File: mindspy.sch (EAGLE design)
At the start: 39 parts, among them IC1 ADS1298, IC2 TPS7A4901, X1 DF9-31S, X2 STELLARIS-LAUNCHPADSTELLARIS-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

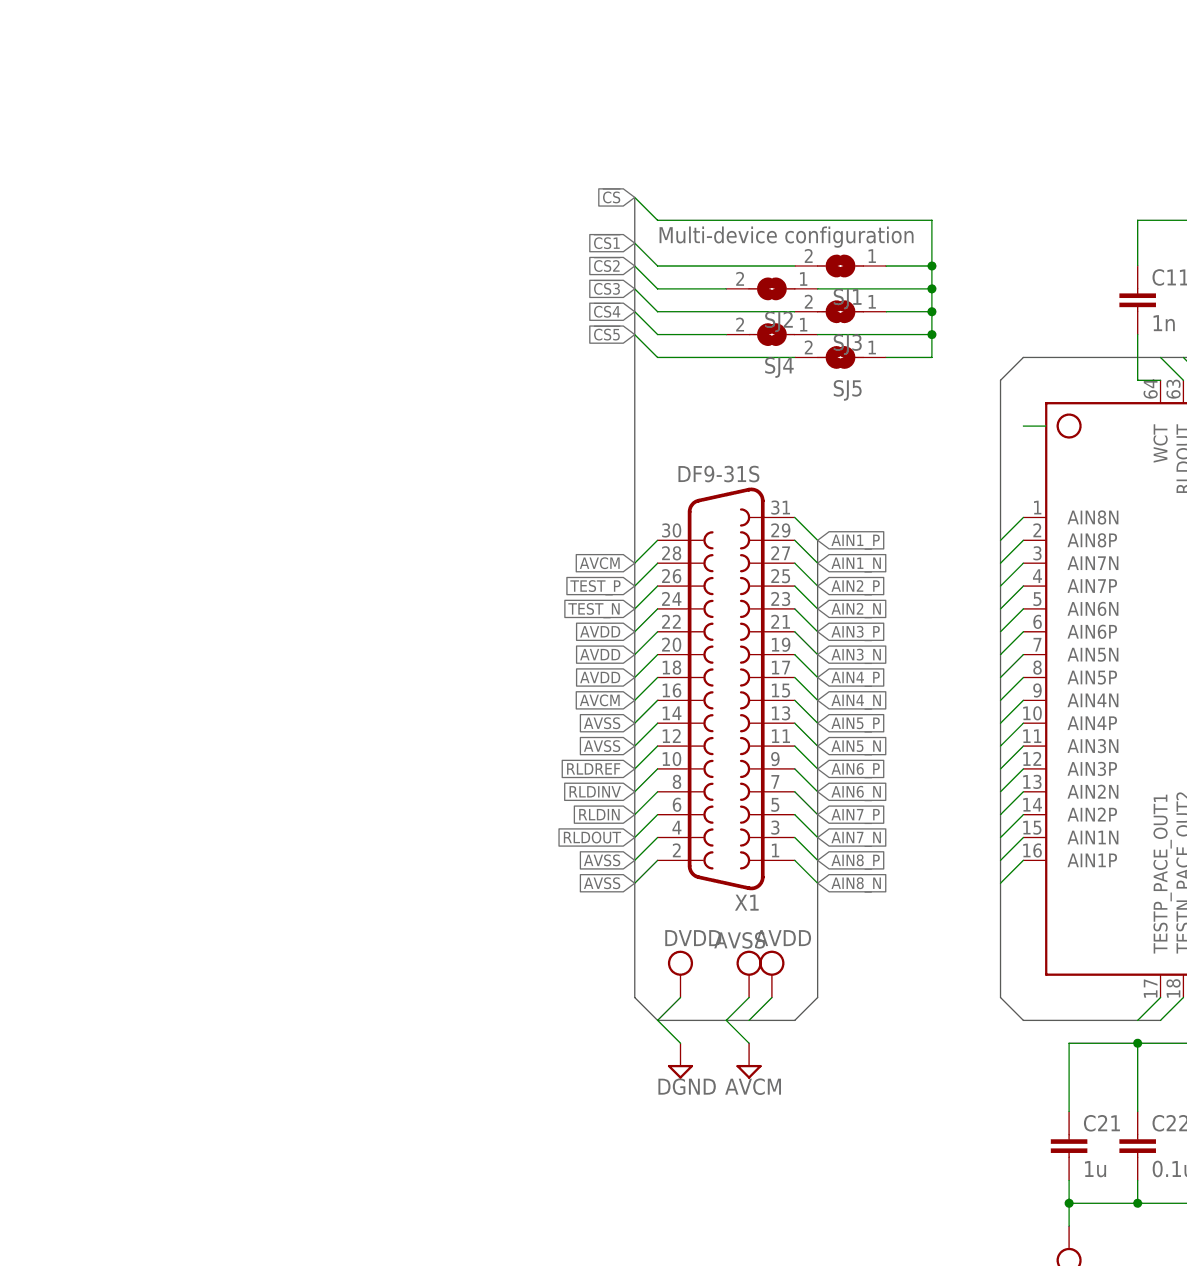
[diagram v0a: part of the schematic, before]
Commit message: almost final
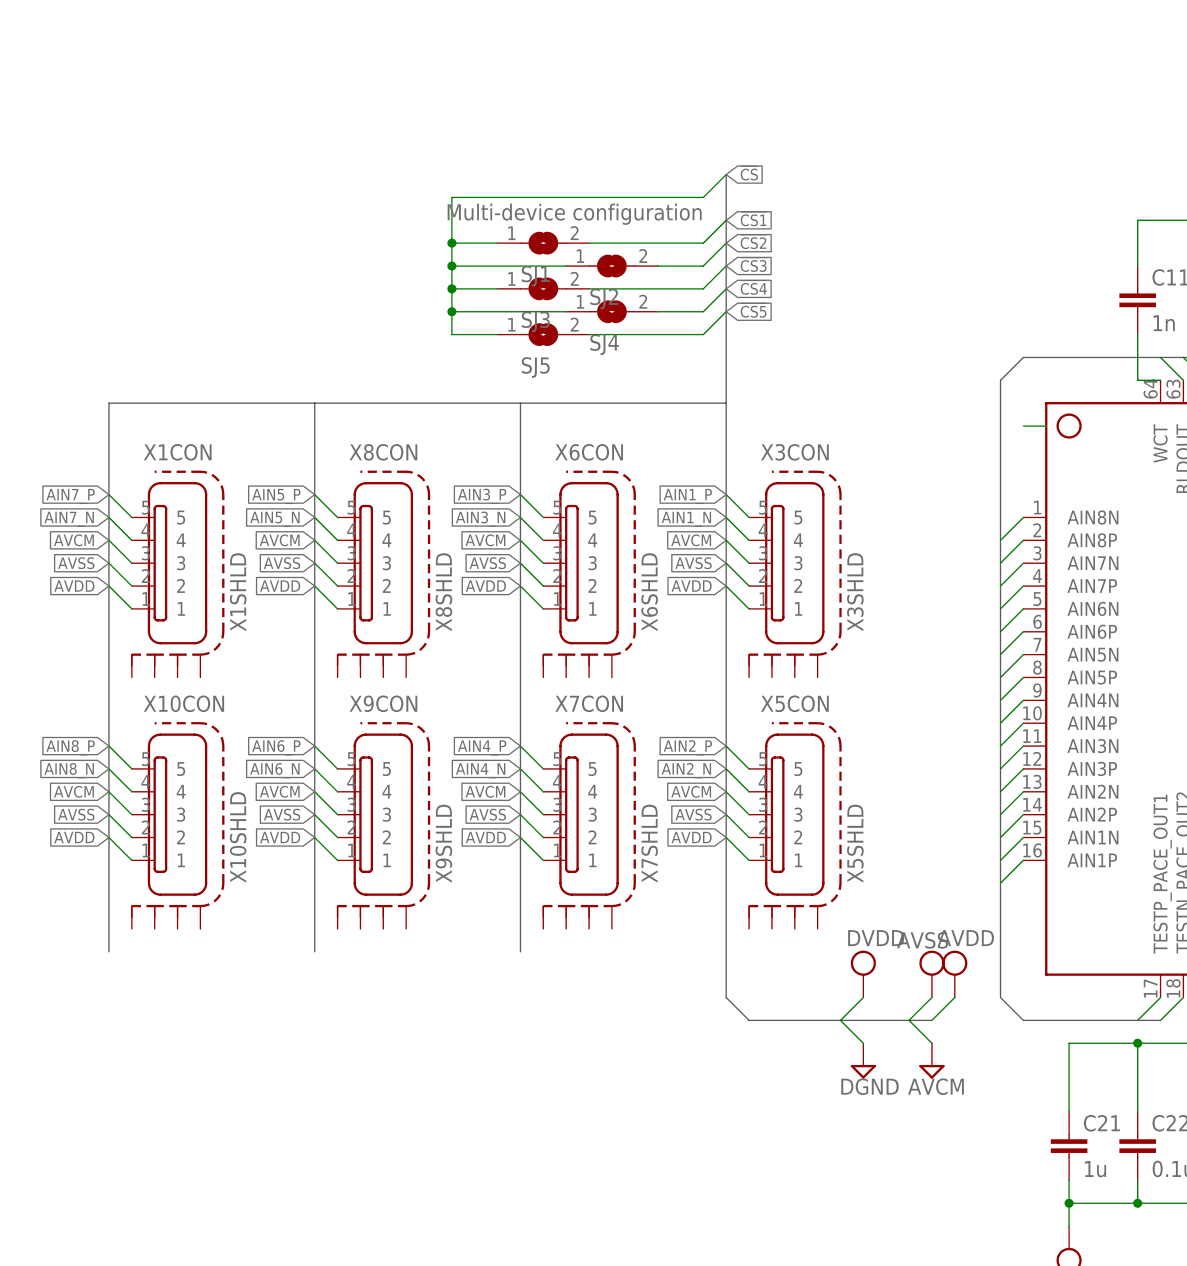
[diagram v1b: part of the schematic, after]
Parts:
- added X10, X3, X5, X6, X7, X8, X9: MICRO-USB-AB-SCHIELD, molex:MICRO-USB-AB-SCHIELD
- X1: value DF9-31S -> MICRO-USB-AB-SCHIELD; device con-hirose:DF9-31S -> molex:MICRO-USB-AB-SCHIELD
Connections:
- net AIN1_N: now also X3CON.4; no longer X1.29
- net AIN1_P: now also X3CON.5; no longer X1.31
- net AIN2_N: now also X5CON.4; no longer X1.25
- net AIN2_P: now also X5CON.5; no longer X1.27
- net AIN3_N: now also X6CON.4; no longer X1.21
- net AIN3_P: now also X6CON.5; no longer X1.23
- net AIN4_N: now also X7CON.4; no longer X1.17
- net AIN4_P: now also X7CON.5; no longer X1.19
- net AIN5_N: now also X8CON.4; no longer X1.13
- net AIN5_P: now also X8CON.5; no longer X1.15
- net AIN6_N: now also X9CON.4; no longer X1.9
- net AIN6_P: now also X9CON.5; no longer X1.11
- net AIN7_N: now also X1CON.4; no longer X1.5
- net AIN7_P: now also X1CON.5; no longer X1.7
- net AIN8_N: now also X10CON.4; no longer X1.1
- net AIN8_P: now also X10CON.5; no longer X1.3
- net AVCM: now also X10CON.3, X1CON.3, X3CON.3, X5CON.3, X6CON.3, X7CON.3, X8CON.3, X9CON.3; no longer X1.18, X1.30
- net AVDD: now also X10CON.1, X1CON.1, X3CON.1, X5CON.1, X6CON.1, X7CON.1, X8CON.1, X9CON.1; no longer X1.20, X1.22, X1.24
- net AVSS: now also X10CON.2, X1CON.2, X3CON.2, X5CON.2, X6CON.2, X7CON.2, X8CON.2, X9CON.2; no longer X1.14, X1.16, X1.2, X1.4
- net RLDIN: no longer X1.8
- net RLDINV: no longer X1.10
- net RLDOUT: no longer X1.6
- net RLDREF: no longer X1.12
- net TEST_N: no longer X1.26
- net TEST_P: no longer X1.28
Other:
- moved on the sheet: SJ1, SJ2, SJ3, SJ4, SJ5

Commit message: errorneous previous commit
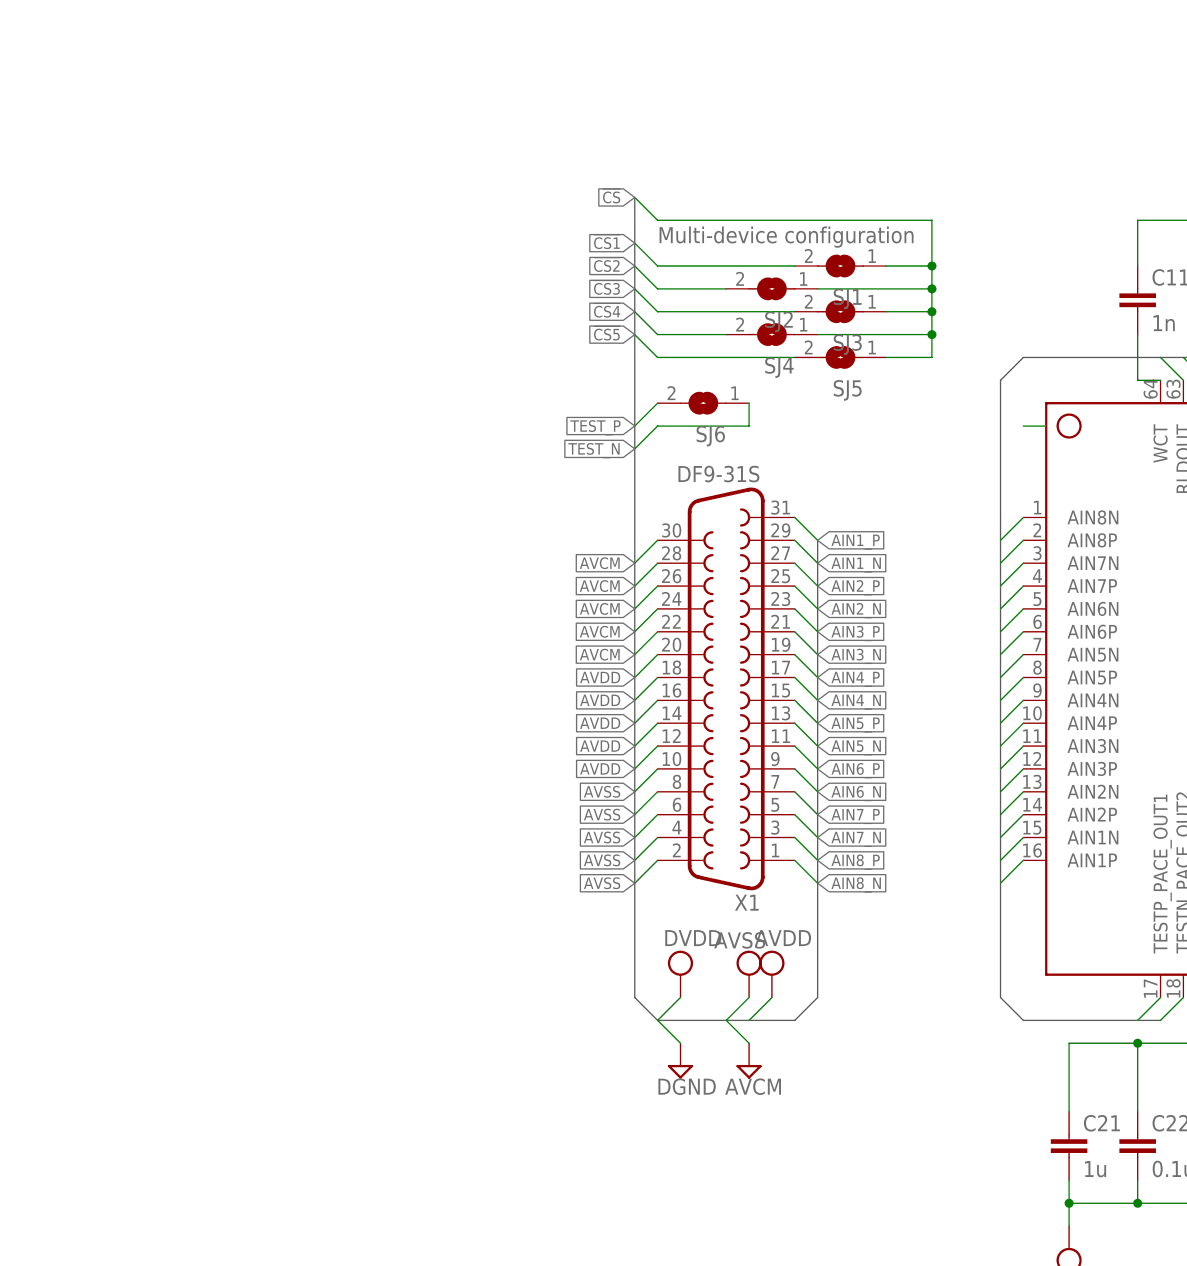
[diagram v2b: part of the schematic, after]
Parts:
- removed X10, X3, X5, X6, X7, X8, X9: MICRO-USB-AB-SCHIELD, molex:MICRO-USB-AB-SCHIELD
- added SJ6: (no value), jumper:SJ
- X1: value MICRO-USB-AB-SCHIELD -> DF9-31S; device molex:MICRO-USB-AB-SCHIELD -> con-hirose:DF9-31S
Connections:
- net AIN1_N: now also X1.29; no longer X3CON.4
- net AIN1_P: now also X1.31; no longer X3CON.5
- net AIN2_N: now also X1.25; no longer X5CON.4
- net AIN2_P: now also X1.27; no longer X5CON.5
- net AIN3_N: now also X1.21; no longer X6CON.4
- net AIN3_P: now also X1.23; no longer X6CON.5
- net AIN4_N: now also X1.17; no longer X7CON.4
- net AIN4_P: now also X1.19; no longer X7CON.5
- net AIN5_N: now also X1.13; no longer X8CON.4
- net AIN5_P: now also X1.15; no longer X8CON.5
- net AIN6_N: now also X1.9; no longer X9CON.4
- net AIN6_P: now also X1.11; no longer X9CON.5
- net AIN7_N: now also X1.5; no longer X1CON.4
- net AIN7_P: now also X1.7; no longer X1CON.5
- net AIN8_N: now also X1.1; no longer X10CON.4
- net AIN8_P: now also X1.3; no longer X10CON.5
- net AVCM: now also X1.22, X1.24, X1.26, X1.28, X1.30; no longer X10CON.3, X1CON.3, X3CON.3, X5CON.3, X6CON.3, X7CON.3, X8CON.3, X9CON.3
- net AVDD: now also X1.12, X1.14, X1.16, X1.18, X1.20; no longer X10CON.1, X1CON.1, X3CON.1, X5CON.1, X6CON.1, X7CON.1, X8CON.1, X9CON.1
- net AVSS: now also X1.10, X1.2, X1.4, X1.6, X1.8; no longer X10CON.2, X1CON.2, X3CON.2, X5CON.2, X6CON.2, X7CON.2, X8CON.2, X9CON.2
- net TEST_N: now also SJ6.1
- net TEST_P: now also SJ6.2
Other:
- moved on the sheet: SJ1, SJ2, SJ3, SJ4, SJ5
